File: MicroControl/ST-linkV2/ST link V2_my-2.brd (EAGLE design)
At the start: 48.9 x 22.5 mm, 38 parts, among them IC1 LD117-3.3, Q1 8000 kHz, U1 STM32F103CBT6, X2 CON-PH12-EDGE

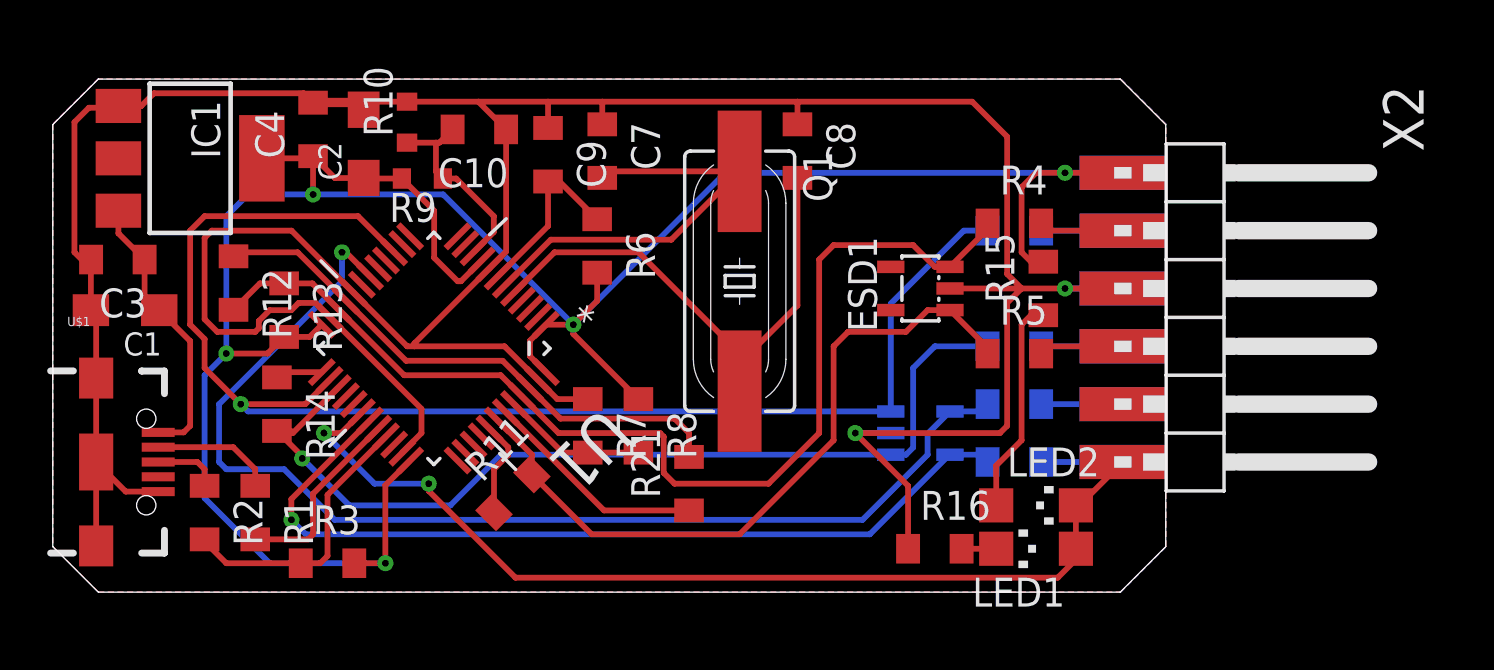
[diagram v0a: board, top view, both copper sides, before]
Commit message: _
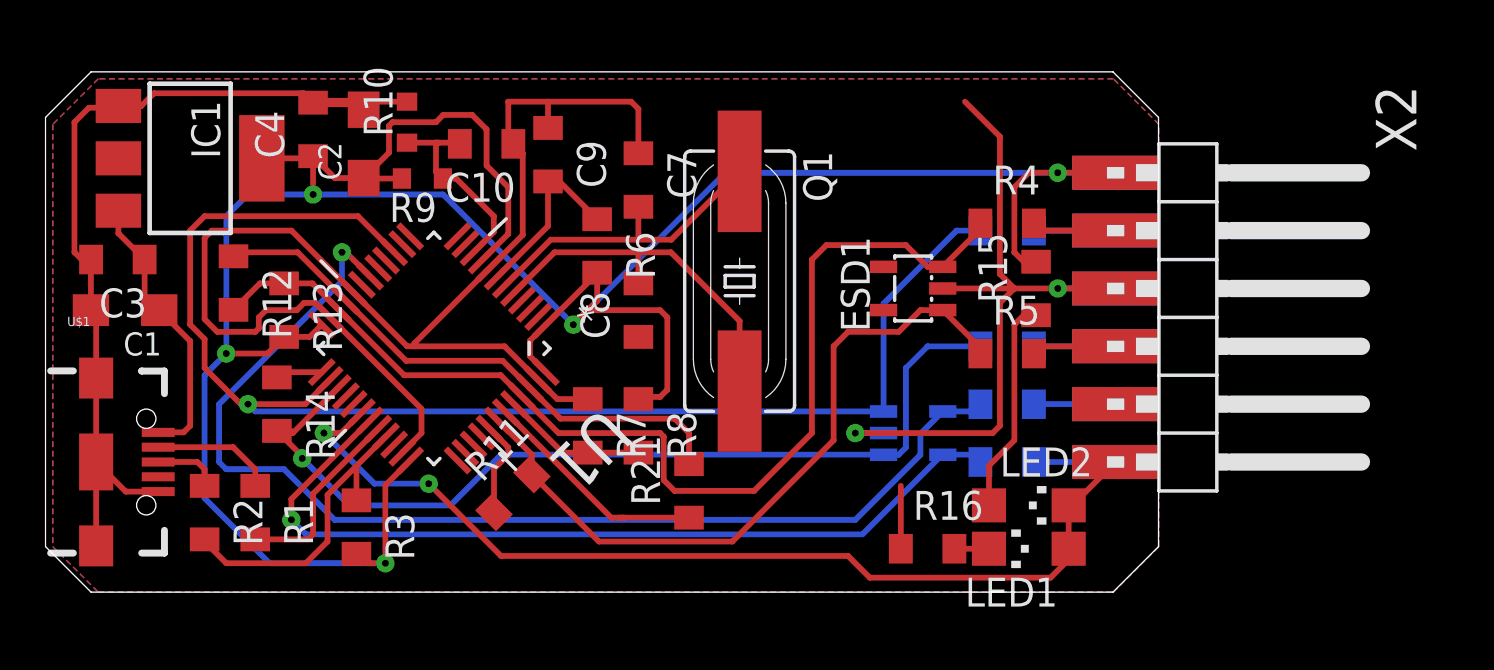
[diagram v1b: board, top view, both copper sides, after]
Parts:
- moved C8 9.88 mm to (25.7, 12.1), turned to 90 degrees
- moved C7 2.03 mm to (25.7, 17.8)
- moved R3 2.03 mm to (13.3, 2.54), turned to 270 degrees
- moved C10 0.71 mm to (19.1, 19.4)
- moved ESD1 0.32 mm to (37.8, 13.0)
- moved ESD2 0.32 mm to (37.8, 6.67)
- moved LED1 0.32 mm to (42.9, 1.59)
- moved LED2 0.32 mm to (42.9, 3.49)
- moved R15 0.32 mm to (43.2, 13.0)
- moved R16 0.32 mm to (38.4, 1.59)
- moved R17 0.32 mm to (41.9, 15.6)
- moved R18 0.32 mm to (41.9, 10.5)
- moved R19 0.32 mm to (41.9, 7.94)
- moved R20 0.32 mm to (41.9, 5.40)
- moved R4 0.32 mm to (41.9, 15.9)
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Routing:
- net GND: track 157.5 -> 134.8 mm
- net +3V3: track 112.8 -> 126.8 mm
- net N$6: track 26.0 -> 16.7 mm
- net N$7: track 18.5 -> 13.8 mm
- net USB_D+: track 12.3 -> 13.4 mm
- net T_SWCLK: track 61.8 -> 61.1 mm
- net U1_BL_TX: track 43.4 -> 42.9 mm
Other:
- board size 48.9 x 22.5 mm -> 48.9 x 22.8 mm
